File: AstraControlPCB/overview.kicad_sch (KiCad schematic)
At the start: 0 parts

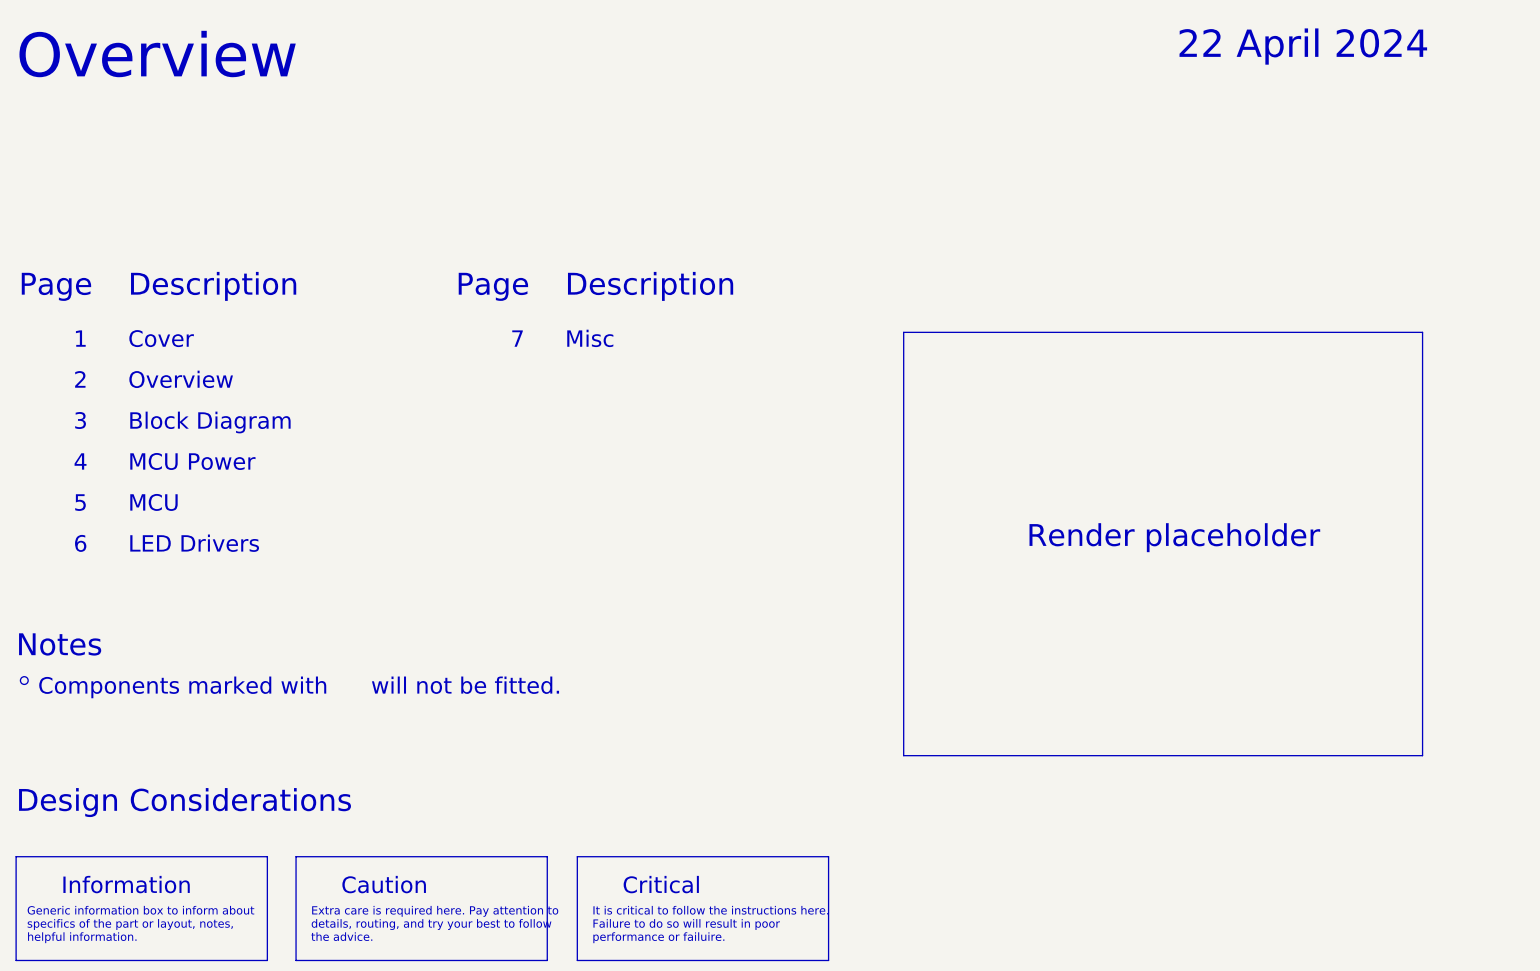
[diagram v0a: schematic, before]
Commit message: workflow
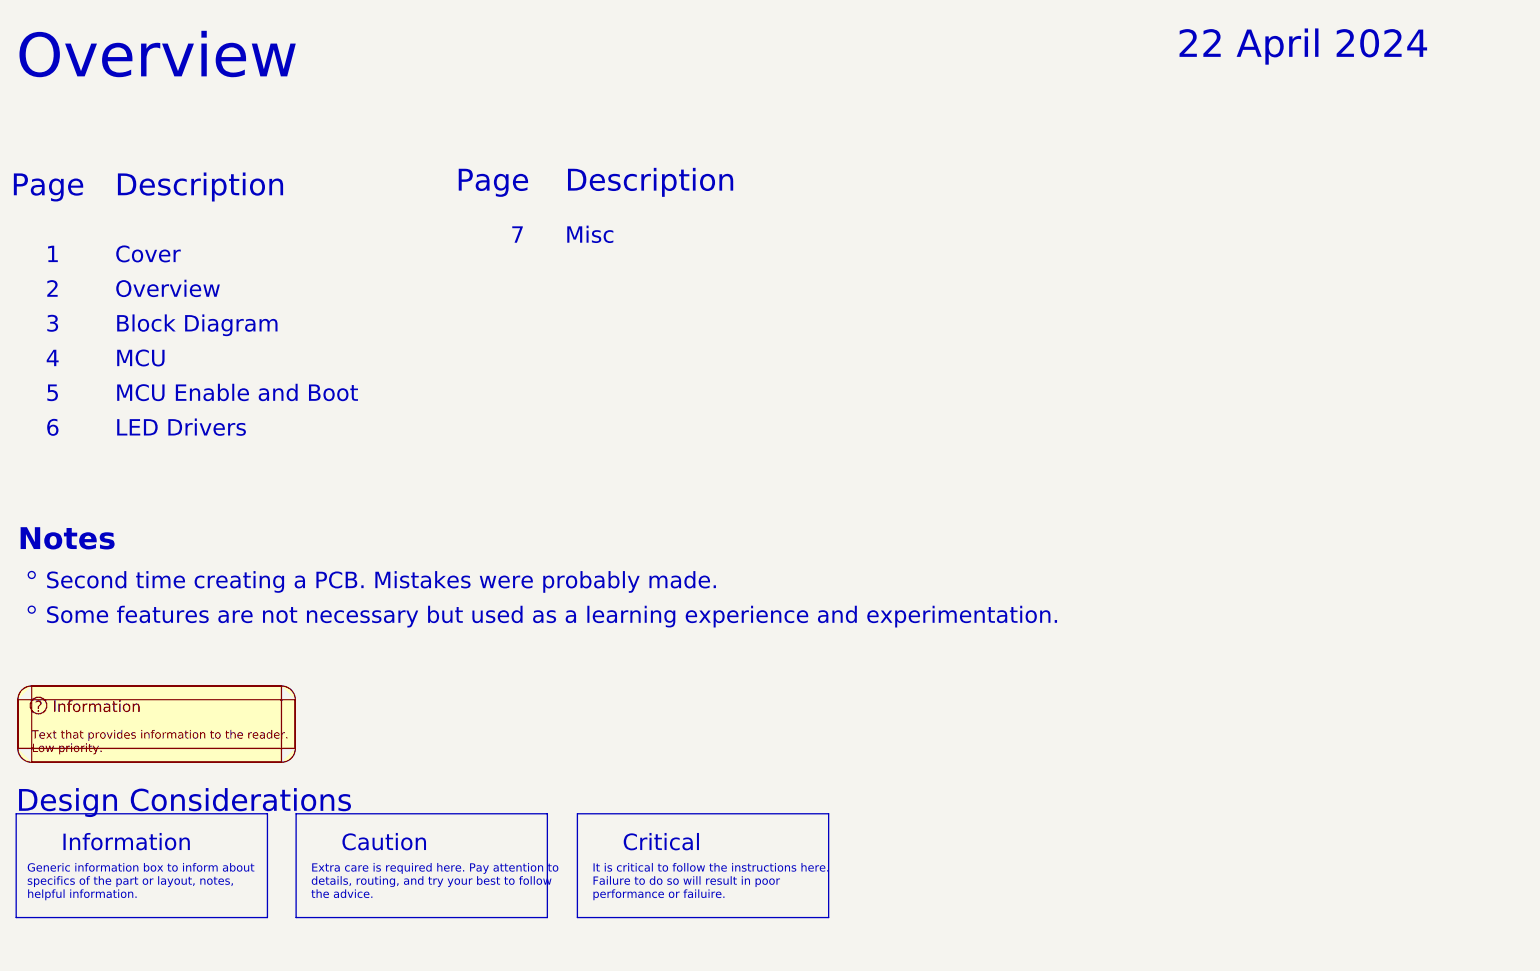
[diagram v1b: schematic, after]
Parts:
- added I2: ~, symbol LiveAstra:Information_Box
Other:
- note added: "MCU Enable and Boot"
- note added: "Second time creating a PCB. Mistakes were probably made."
- note added: "Some features are not necessary but used as a learning experience and experimentation."
- note removed: "Components marked with will not be fitted."
- note removed: "MCU Power"
- note removed: "Render placeholder"
